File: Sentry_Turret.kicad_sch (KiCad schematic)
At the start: 38 parts, among them J14 501645-1620, J16 172298-1108

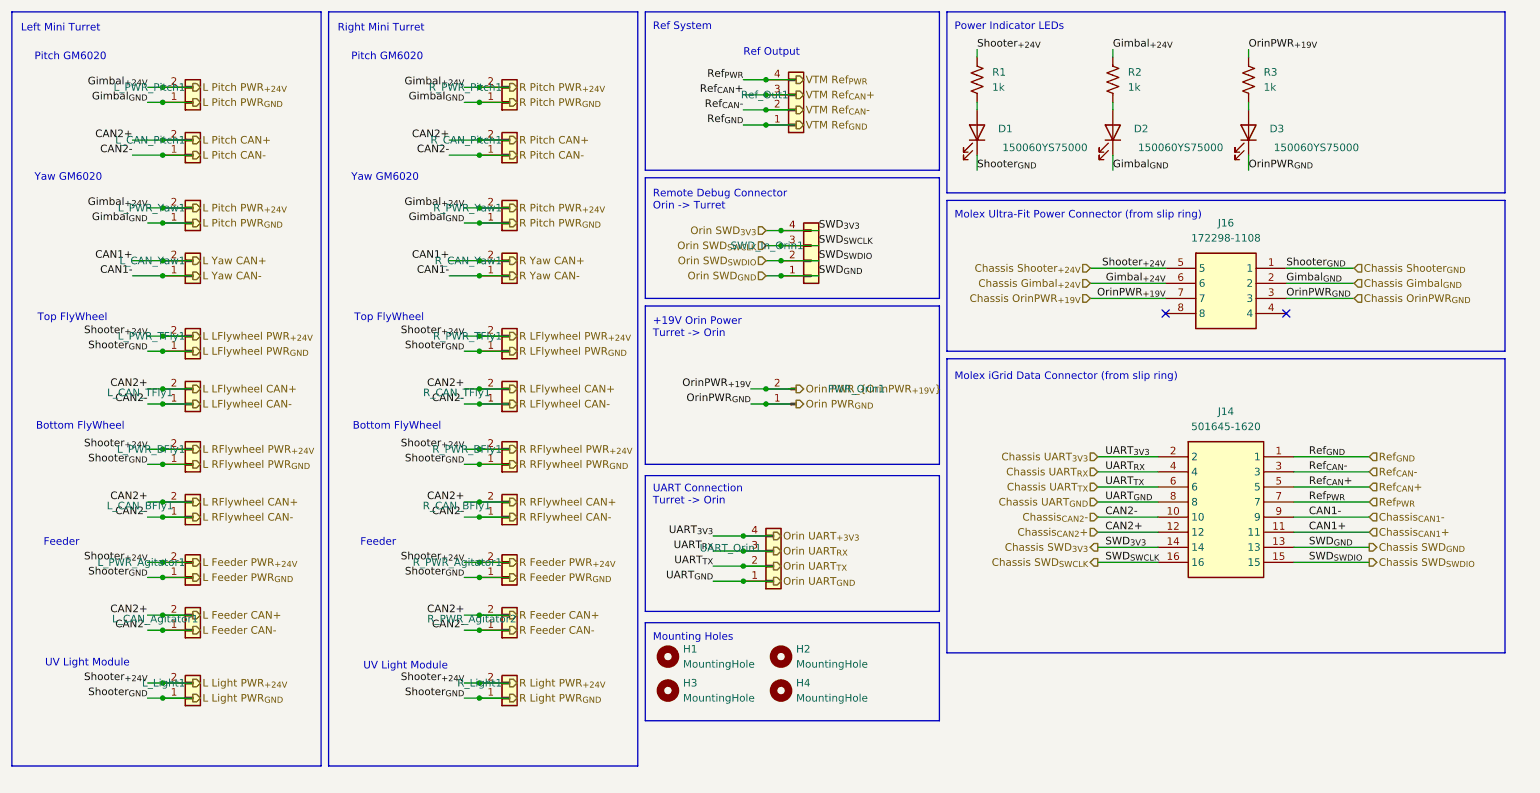
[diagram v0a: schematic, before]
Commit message: Layout review
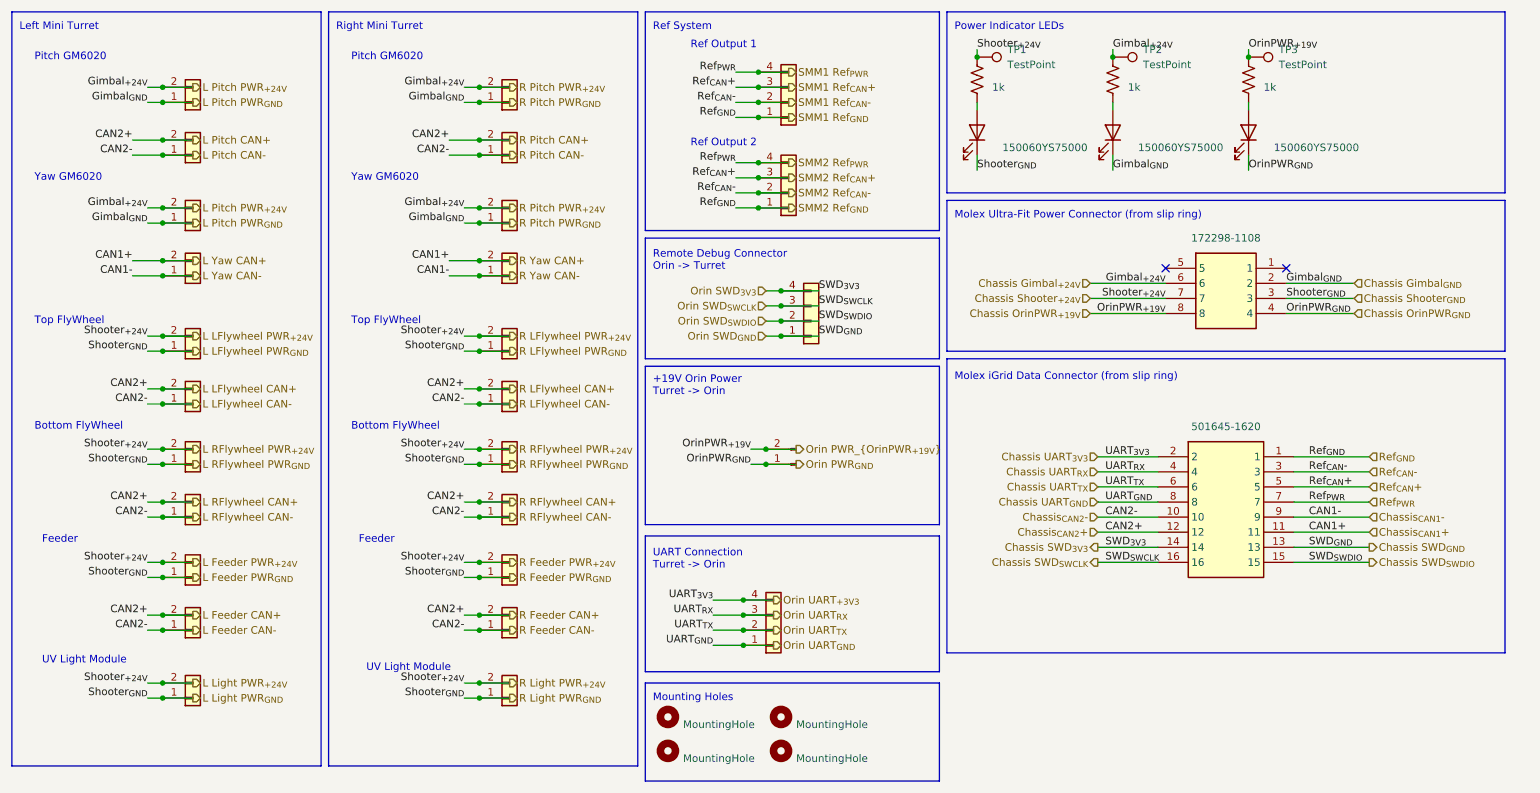
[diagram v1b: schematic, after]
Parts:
- added Ref_Out2: Conn_01x04_Pin, Connector_JST:JST_GH_BM04B-GHS-TBT_1x04-1MP_P1.25mm_Vertical, symbol Connector_Generic:Conn_01x04
- added TP1, TP2, TP3: TestPoint, TestPoint:TestPoint_2Pads_Pitch2.54mm_Drill0.8mm, symbol Connector:TestPoint
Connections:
- net Chassis Gimbal_{+24V}: now also TP2.1
- net Chassis OrinPWR_{+19V}: now also J16.8, TP3.1; no longer J16.7
- net Chassis OrinPWR_{GND}: now also J16.4; no longer J16.3
- net Chassis Shooter_{+24V}: now also J16.7, TP1.1; no longer J16.5
- net Chassis Shooter_{GND}: now also J16.3; no longer J16.1
- net Ref_{CAN}+: now also Ref_Out2.3 (Pin_3)
- net Ref_{CAN}-: now also Ref_Out2.2 (Pin_2)
- net Ref_{GND}: now also Ref_Out2.1 (Pin_1)
- net Ref_{PWR}: now also Ref_Out2.4 (Pin_4)
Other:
- note added: "Ref Output 1"
- note added: "Ref Output 2"
- note removed: "Ref Output"
